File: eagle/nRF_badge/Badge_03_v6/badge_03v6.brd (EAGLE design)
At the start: 30 x 70 mm, 45 parts, among them U1 LIS2DH12, U2 LP2985LV, U3 MCP6231, U5 M95M02, Y1 32768Hz

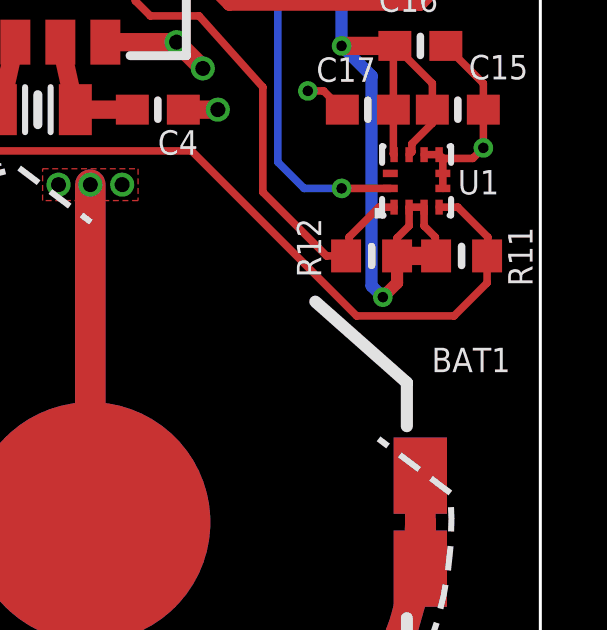
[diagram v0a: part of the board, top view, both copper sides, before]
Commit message: Exporting gerber and pnp
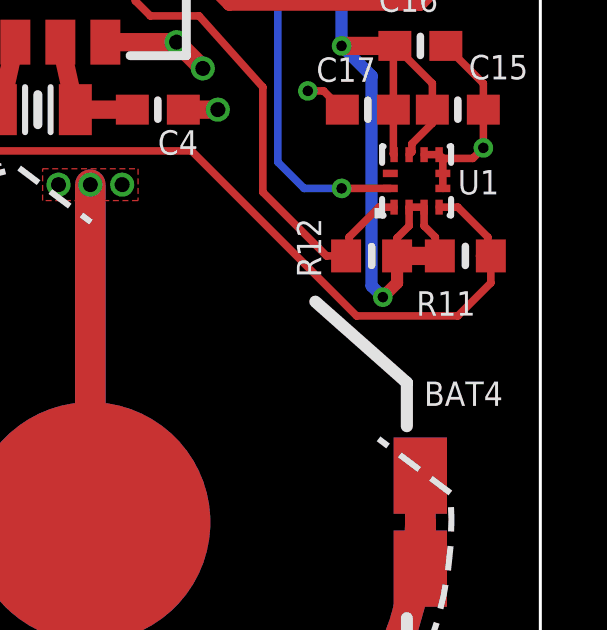
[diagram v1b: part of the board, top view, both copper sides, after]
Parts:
- moved R11 0.12 mm to (27.5, 21.1)
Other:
- board text added: "BAT4"
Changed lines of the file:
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@@
 <rectangle x1="5.25" y1="50.125" x2="6.25" y2="51.5" layer="42"/>
 <text x="9.011" y="33.751" size="1.9304" layer="22" font="vector" ratio="16" rot="MR90" align="top-left">03v6</text>
+<text x="26.125" y="16.125" size="0.8128" layer="25" font="vector" ratio="16">BAT4</text>
 </plain>
 <attributes>
@@
 <attribute name="VALUE" x="8.875" y="58" size="0.8128" layer="27" font="vector" ratio="16"/>
 </element>
-<element name="BAT1" library="Badge" package="BATTCON_20MM_4LEGS_ISO_NOCREAM" value="CR2032" x="15" y="12.25" smashed="yes">
-<attribute name="NAME" x="26.375" y="17.25" size="0.8128" layer="25" font="vector" ratio="16"/>
-</element>
+<element name="BAT1" library="Badge" package="BATTCON_20MM_4LEGS_ISO_NOCREAM" value="CR2032" x="15" y="12.25" smashed="yes"/>
 <element name="C1" library="rcl" package="C1206" value="100u" x="23" y="41.5" smashed="yes">
 <attribute name="NAME" x="19.25" y="41.5" size="0.8128" layer="25" font="vector" ratio="16"/>
@@
 <attribute name="VALUE" x="25.28" y="42.615" size="0.8128" layer="27" font="vector" ratio="16" rot="R90"/>
 </element>
-<element name="BAT4" library="Badge" package="BU2032SM_CREAM" value="CR2032" x="15" y="12.25" rot="R323"/>
+<element name="BAT4" library="Badge" package="BU2032SM_CREAM" value="CR2032" x="15" y="12.25" smashed="yes" rot="R323"/>
 <element name="MIC_F" library="Badge" package="TESTPOINT" value="" x="23.375" y="59"/>
 <element name="M_VCC" library="Badge" package="TESTPOINT" value="" x="26.125" y="44.625"/>
@@
 <attribute name="VALUE" x="21.845" y="26.385" size="0.8128" layer="27" font="vector" ratio="16" rot="R270"/>
 </element>
-<element name="R11" library="rcl" package="R0603" value="1k" x="27.375" y="21.125" smashed="yes">
-<attribute name="NAME" x="29.74" y="20.115" size="0.8128" layer="25" font="vector" ratio="16" rot="R90"/>
-<attribute name="VALUE" x="27.74" y="19.095" size="0.8128" layer="27" font="vector" ratio="16"/>
+<element name="R11" library="rcl" package="R0603" value="1k" x="27.5" y="21.125" smashed="yes">
+<attribute name="NAME" x="25.865" y="19.135" size="0.8128" layer="25" font="vector" ratio="16"/>
+<attribute name="VALUE" x="28.365" y="19.135" size="0.8128" layer="27" font="vector" ratio="16"/>
 </element>
 <element name="R12" library="rcl" package="R0603" value="1k" x="24.375" y="21.125" smashed="yes" rot="R180">
@@
 <wire x1="26.125" y1="22.125" x2="26.5" y2="21.75" width="0.254" layer="1"/>
 <wire x1="26.5" y1="21.75" x2="26.5" y2="21.15" width="0.254" layer="1"/>
-<wire x1="26.525" y1="21.125" x2="26.5" y2="21.15" width="0.254" layer="1"/>
+<wire x1="26.65" y1="21.125" x2="26.5" y2="21.15" width="0.254" layer="1"/>
 <wire x1="25.1" y1="24.525" x2="25.1" y2="26" width="0.254" layer="1"/>
 <wire x1="25.125" y1="24.5" x2="25.1" y2="24.525" width="0.254" layer="1"/>
@@
 <wire x1="25.15" y1="28.125" x2="23.375" y2="28.125" width="0.6096" layer="1"/>
 <via x="24.75" y="19.75" extent="1-16" drill="0.35"/>
-<wire x1="25.225" y1="21.125" x2="26.525" y2="21.125" width="0.6096" layer="1"/>
+<wire x1="25.225" y1="21.125" x2="26.65" y2="21.125" width="0.6096" layer="1"/>
 <wire x1="21" y1="34.875" x2="23.375" y2="32.5" width="0.4064" layer="16"/>
 <wire x1="23.375" y1="32.5" x2="23.375" y2="28.125" width="0.4064" layer="16"/>
@@
 <wire x1="27.25" y1="22.75" x2="28.25" y2="21.75" width="0.254" layer="1"/>
 <wire x1="28.25" y1="21.75" x2="28.25" y2="21.15" width="0.254" layer="1"/>
-<wire x1="28.25" y1="21.15" x2="28.225" y2="21.125" width="0.254" layer="1"/>
-<wire x1="28.225" y1="21.125" x2="27.97013125" y2="21.125" width="0.254" layer="1"/>
-<wire x1="28.225" y1="20.225" x2="28.225" y2="21.125" width="0.254" layer="1"/>
+<wire x1="28.25" y1="21.15" x2="28.35" y2="21.125" width="0.254" layer="1"/>
+<wire x1="28.35" y1="21.125" x2="27.97013125" y2="21.125" width="0.254" layer="1"/>
+<wire x1="28.35" y1="20.225" x2="28.35" y2="21.125" width="0.254" layer="1"/>
 <wire x1="11.14823125" y1="24.77323125" x2="11.2964625" y2="24.625" width="0.254" layer="1"/>
 <wire x1="11.2964625" y1="24.625" x2="18.375" y2="24.625" width="0.254" layer="1"/>
-<wire x1="23.875" y1="19.125" x2="27.125" y2="19.125" width="0.254" layer="1"/>
+<wire x1="23.875" y1="19.125" x2="27.25" y2="19.125" width="0.254" layer="1"/>
 <wire x1="18.375" y1="24.625" x2="23.875" y2="19.125" width="0.254" layer="1"/>
-<wire x1="27.125" y1="19.125" x2="28.225" y2="20.225" width="0.254" layer="1"/>
+<wire x1="27.25" y1="19.125" x2="28.35" y2="20.225" width="0.254" layer="1"/>
 </signal>
 <signal name="CS">
